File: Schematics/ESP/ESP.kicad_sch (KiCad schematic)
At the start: 28 parts, among them J1 Barrel_Jack, Q1 IRLB8721PBF, Q10 IRLML0030, Q11 IRLML0030, Q12 IRLML0030, Q13 IRLML0030, Q14 IRLML0030, Q2 IRLB8721PBF, Q3 IRLB8721PBF, Q4 IRLB8721PBF, Q5 IRLB8721PBF, Q6 IRLB8721PBF, Q7 IRLB8721PBF, Q8 IRLB8721PBF, Q9 IRLML0030, U1 AP9101CK, U2 AP9101CK, U3 AP9101CK

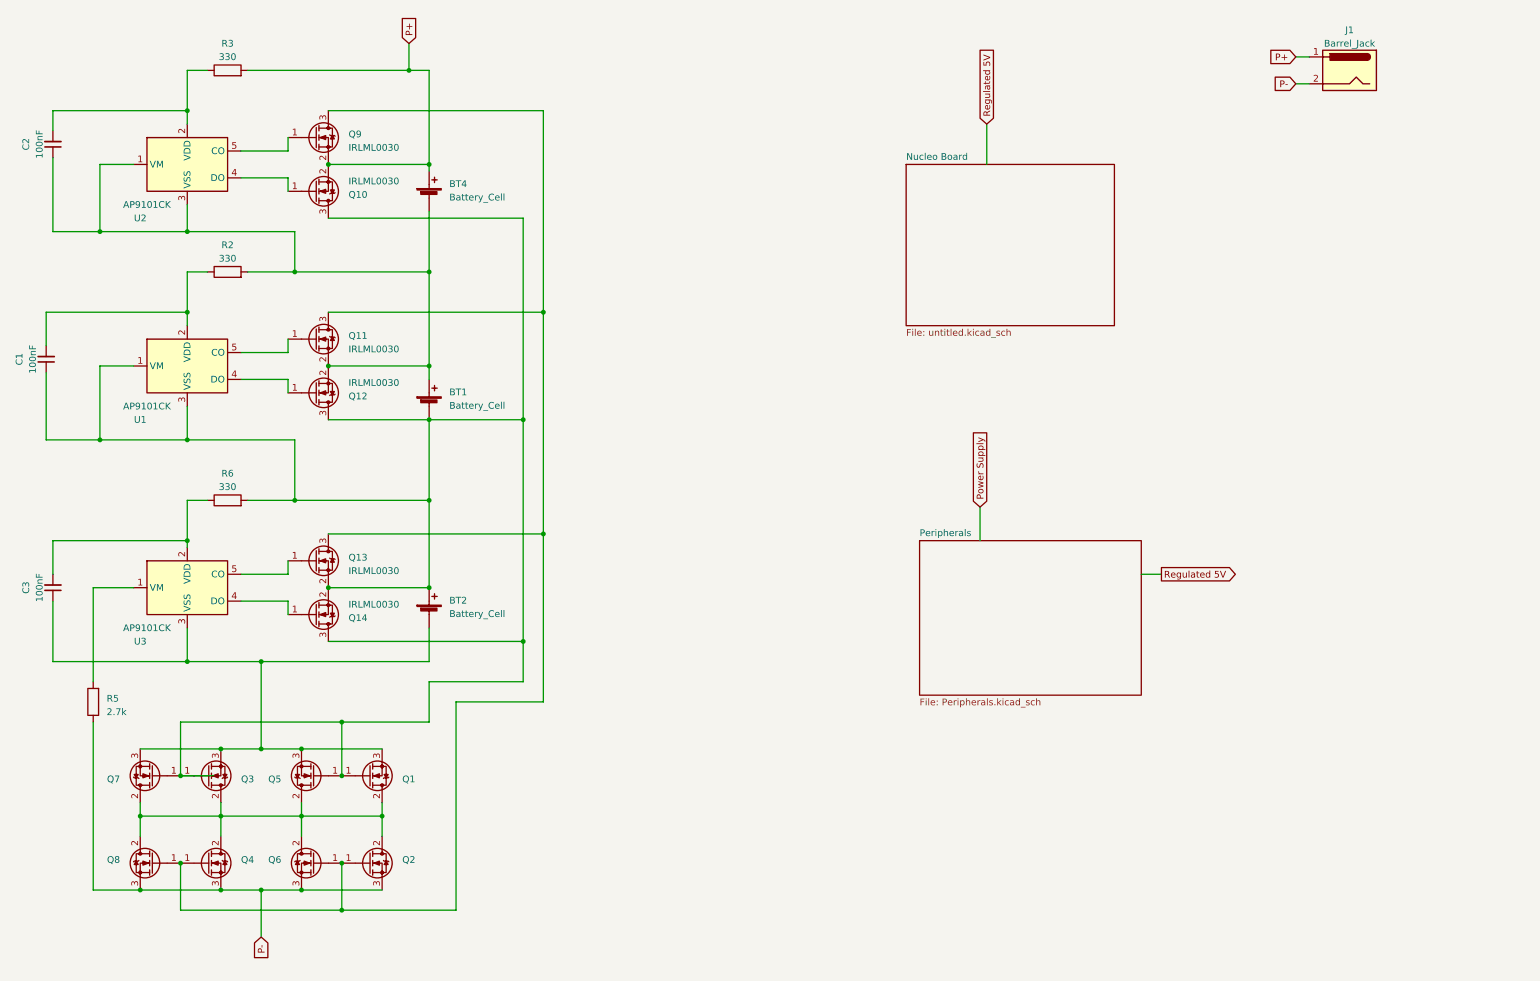
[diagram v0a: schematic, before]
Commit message: Schematics
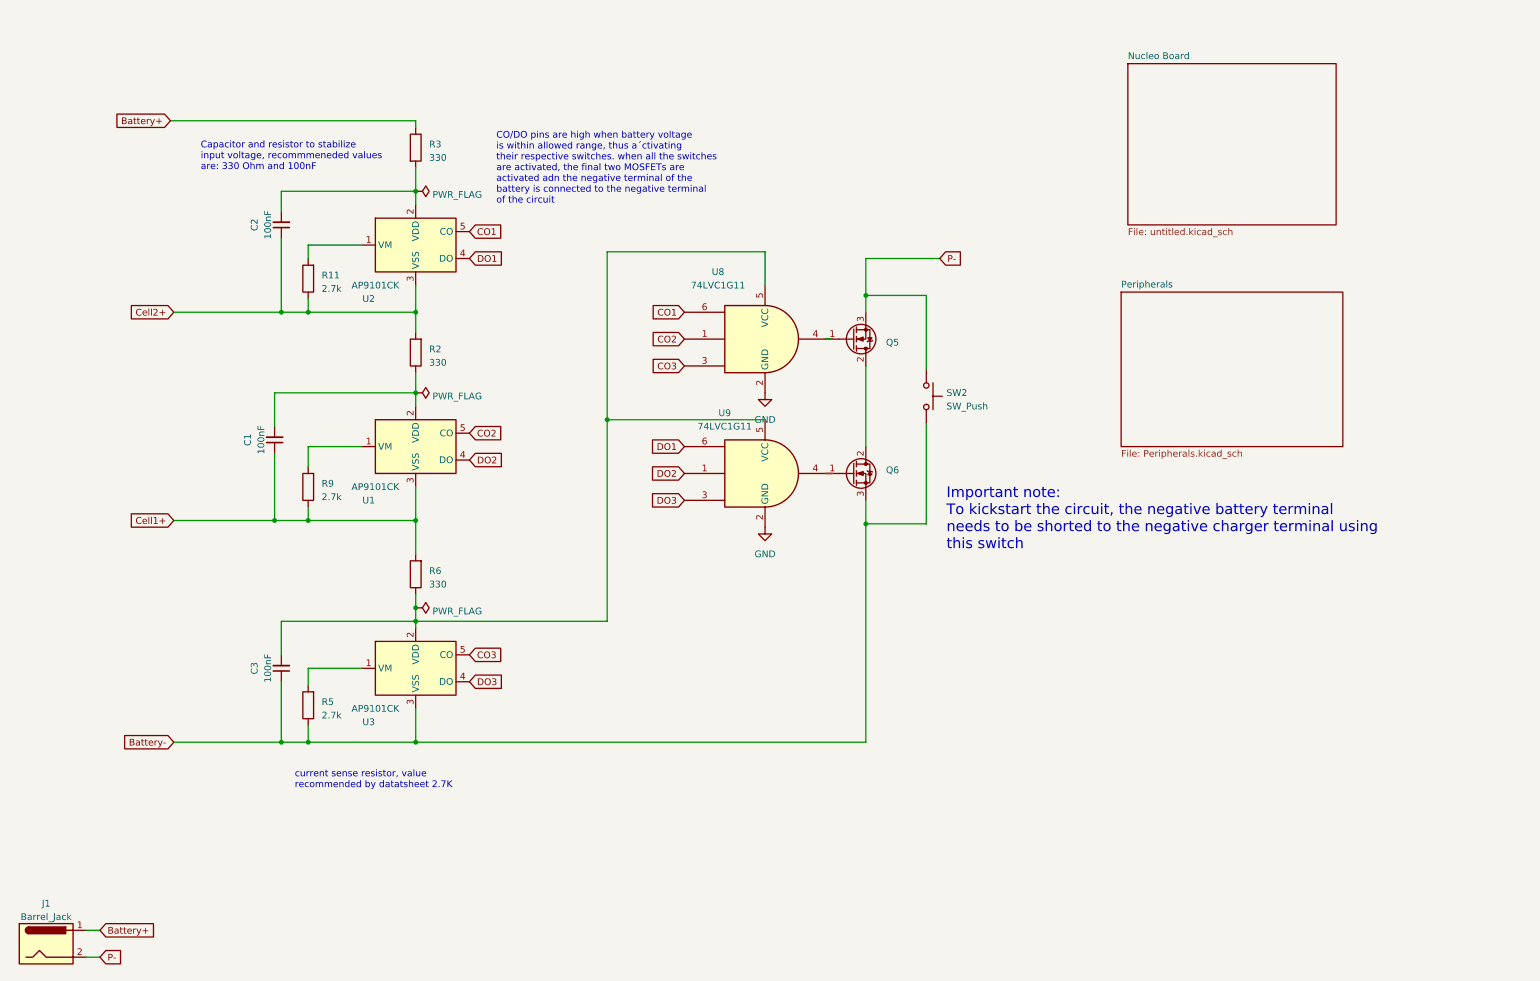
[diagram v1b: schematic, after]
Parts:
- removed BT1, BT2, BT4: Battery_Cell, symbol Device:Battery_Cell
- removed Q1, Q2, Q3, Q4, Q7, Q8: IRLB8721PBF, Package_TO_SOT_THT:TO-220-3_Vertical, symbol Transistor_FET:IRLB8721PBF
- removed Q10, Q11, Q12, Q13, Q14, Q9: IRLML0030, Package_TO_SOT_SMD:SOT-23, symbol Transistor_FET:IRLML0030
- added R11, R9: 2.7k, Resistor_SMD:R_1206_3216Metric_Pad1.30x1.75mm_HandSolder, symbol Device:R
- added SW2: SW_Push, Button_Switch_SMD:SW_SPST_PTS645, symbol Switch:SW_Push
- added U8, U9: 74LVC1G11, Package_TO_SOT_SMD:SOT-23-6_Handsoldering, symbol 74xGxx:74LVC1G11
- C1, C2, C3: footprint (none) -> Capacitor_Tantalum_SMD:CP_EIA-7343-31_Kemet-D_Pad2.25x2.55mm_HandSolder
- J1: footprint (none) -> RAPC722X:SWITCHCRAFT_RAPC722X
- Q6: digikey link (none) -> https://www.digikey.fi/en/products/detail/infineon-technolo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
- R2, R3, R5, R6: footprint (none) -> Resistor_SMD:R_1206_3216Metric_Pad1.30x1.75mm_HandSolder
- U2: digikey link (none) -> https://www.digikey.fi/en/products/detail/diodes-incorporat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
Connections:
- net P-: now also Q5.3 (S), SW2.1; no longer Q6.3 (S), R5.1
- net at Q6.1 (G): now also U9.4
- net DO2: now reaches U1.4 (DO)
- net DO2: now also U9.1
- net Cell2+: now reaches C2.1, R2.2, U2.3 (VSS)
- net Cell2+: now also R11.1; no longer U2.1 (VM)
- net Cell1+: now reaches C1.1, R6.2, U1.3 (VSS)
- net Cell1+: now also R9.1; no longer Q5.1 (G), U1.1 (VM)
- net DO1: now reaches U2.4 (DO)
- net DO1: now also U9.6
- net at C2.2, U2.2 (VDD): now also R3.2; no longer R3.1
- net CO2: now reaches U1.5 (CO)
- net CO2: now also U8.1
- net Battery-: now reaches C3.1, U3.3 (VSS)
- net Battery-: now also Q6.3 (S), R5.1, SW2.2; no longer Q5.3 (S)
- net at C3.2, R6.1, U3.2 (VDD): now also U8.5 (VCC), U9.5 (VCC)
- net DO3: now reaches U3.4 (DO)
- net DO3: now also U9.3
- net CO1: now reaches U2.5 (CO)
- net CO1: now also U8.6
- net CO3: now reaches U3.5 (CO)
- net CO3: now also U8.3
- net P+ renamed Battery+
- net Battery+: now also R3.1; no longer R3.2
- new net: R9.2, U1.1 (VM)
- new net: Q5.1 (G), U8.4
- new net: R11.2, U2.1 (VM)
- new net GND: U8.2 (GND), U9.2 (GND)
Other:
- note added: "CO/DO pins are high when battery voltage is within allowed range, thus a´ctivating their respective switches. when all the switches are activated, the final two MOSFETs are activated adn the negative terminal of the battery is connected to the negative terminal of the circuit"
- note added: "Capacitor and resistor to stabilize input voltage, recommmeneded values are: 330 Ohm and 100nF"
- note added: "Important note: To kickstart the circuit, the negative battery terminal needs to be shorted to the negative charger terminal using this switch"
- note added: "current sense resistor, value recommended by datatsheet 2.7K"
- moved on the sheet: C1, C2, C3, J1, Q5, Q6, R2, R5, R6, U1, U2, U3
